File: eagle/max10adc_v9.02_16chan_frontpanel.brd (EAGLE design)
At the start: 79 x 65 mm, 106 parts, among them CN1 8p-2.54, X1 BU-SMA-V, X10 BU-SMA-V, X11 BU-SMA-V, X12 BU-SMA-V, X13 BU-SMA-V, X14 BU-SMA-V, X15 BU-SMA-V, X16 BU-SMA-V, X2 BU-SMA-V, X3 BU-SMA-V, X4 BU-SMA-V, X5 BU-SMA-V, X6 BU-SMA-V, X7 BU-SMA-V, X8 BU-SMA-V, X9 BU-SMA-V

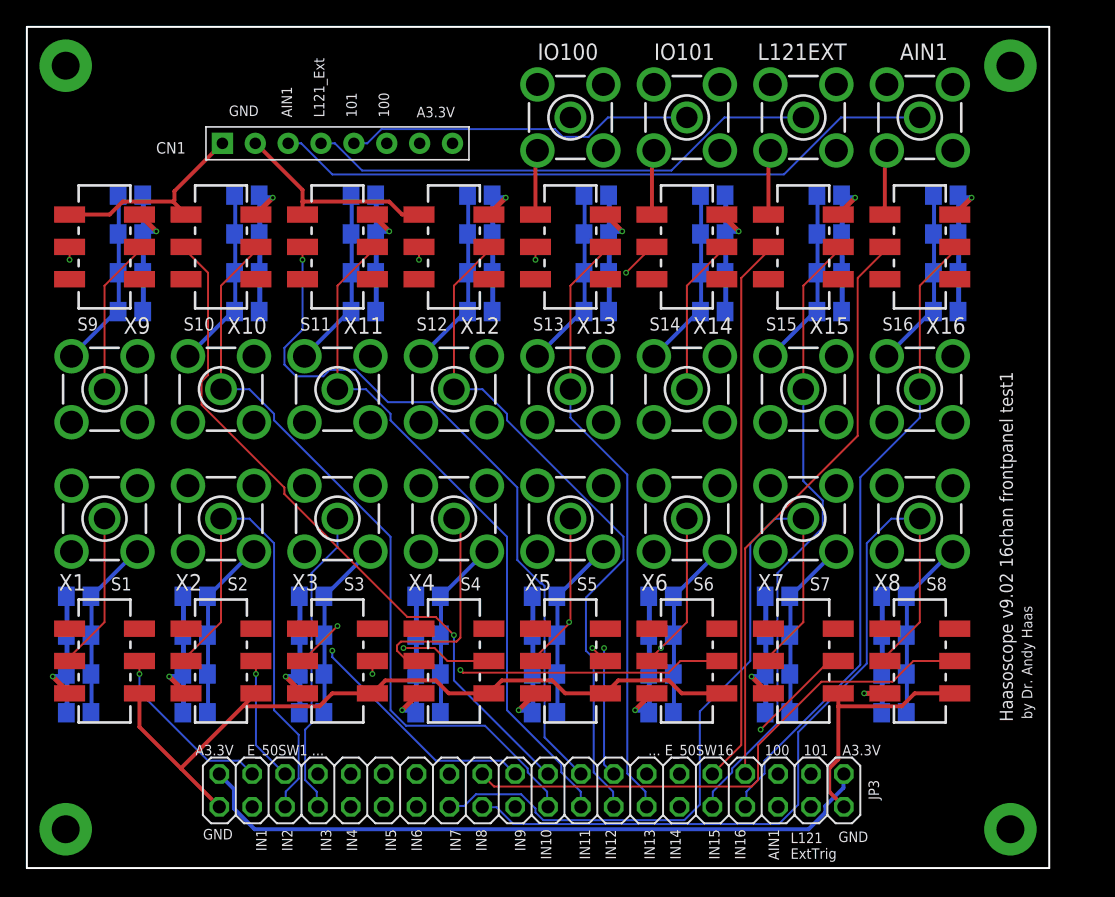
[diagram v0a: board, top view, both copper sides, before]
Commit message: back connectors
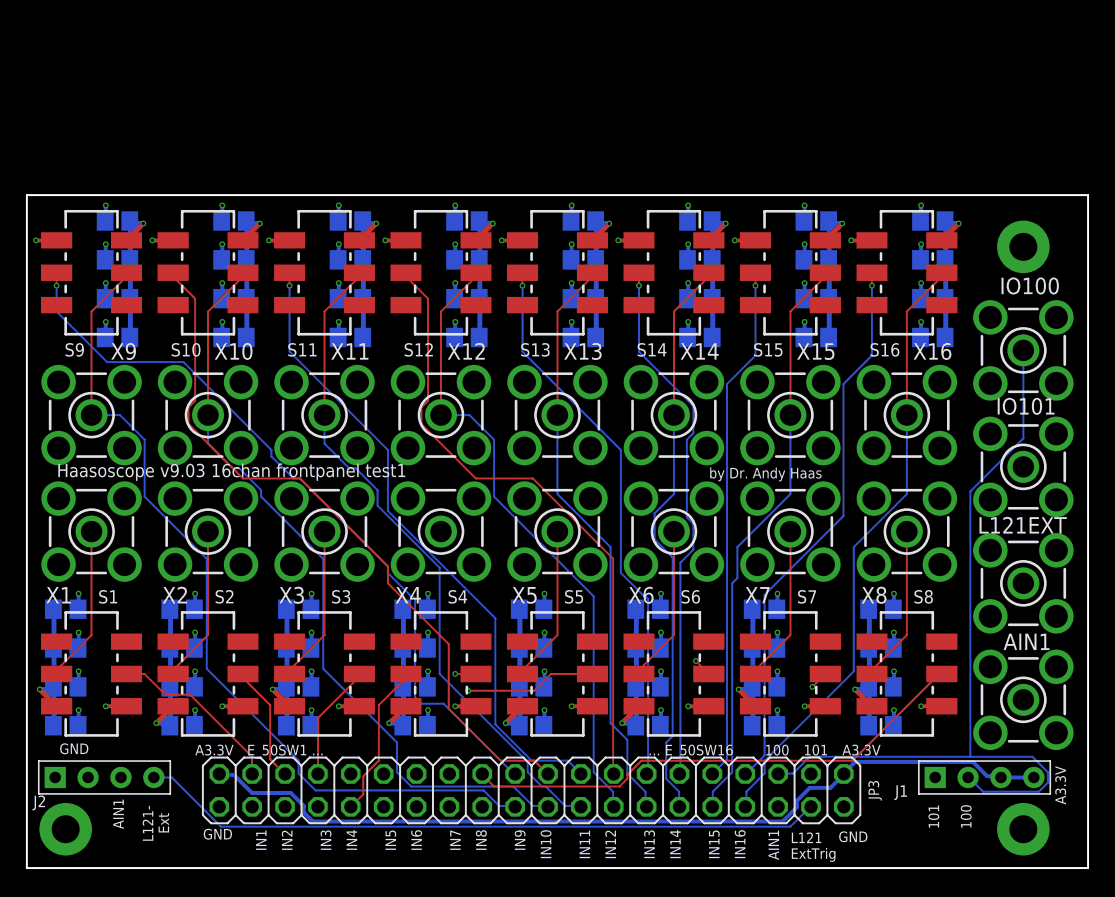
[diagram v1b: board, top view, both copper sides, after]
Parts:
- removed CN1: 8p-2.54, Seeed-Connector:H8-2.54
- removed H1: STANDOFF_ELECTRICAL, SparkFun-Hardware:STANDOFF-ELECTRICAL
- added J1, J2: 4p-2.54, Seeed-Connector:H4-2.54
- moved H2 75.3 mm to (77.0, 48.0)
- moved AIN1 45.7 mm to (77.0, 13.0)
- moved L121EXT 39.8 mm to (77.0, 22.0)
- moved IO100 39.4 mm to (77.0, 40.0)
- moved IO101 37.5 mm to (77.0, 31.0)
- moved R101 2.24 mm to (61.0, 41.0)
- moved R102 2.24 mm to (61.0, 44.0)
- moved R103 2.24 mm to (61.0, 47.0)
- moved R104 2.24 mm to (61.0, 50.0)
- moved R109 2.24 mm to (70.0, 41.0)
- moved R110 2.24 mm to (70.0, 44.0)
- moved R111 2.24 mm to (70.0, 47.0)
- moved R112 2.24 mm to (70.0, 50.0)
- moved R13 2.24 mm to (7.00, 41.0)
- moved R14 2.24 mm to (7.00, 44.0)
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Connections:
- net AIN1: now also J2.3; no longer CN1.3
- net GND: now also J2.1, J2.2; no longer CN1.1, CN1.2, H1.P1
- net IO_100: now also J1.2; no longer CN1.6
- net IO_101: now also J1.1; no longer CN1.5
- net L121: now also J2.4; no longer CN1.4
- net VCCA: now also J1.3, J1.4; no longer CN1.7, CN1.8
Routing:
- net GND: track 359.0 -> 105.6 mm, vias 0 -> 80
- net VCCA: track 111.3 -> 67.5 mm
- net IO_101: track 81.8 -> 38.4 mm
- net AIN1: track 114.1 -> 77.8 mm
- net L121: track 96.3 -> 80.2 mm
- net INJ14: track 55.1 -> 44.2 mm
- net INJ9: track 76.2 -> 65.5 mm
- net INJ7: track 60.1 -> 50.7 mm
- net IO_100: track 72.0 -> 62.7 mm
- net INJ8: track 65.0 -> 55.9 mm
- net E_50SW11: track 56.2 -> 49.7 mm
- net E_50SW13: track 48.4 -> 42.8 mm
- net E_50SW4: track 18.4 -> 12.9 mm
- net INJ4: track 42.6 -> 37.0 mm
- net E_50SW7: track 34.7 -> 40.1 mm
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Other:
- board size 79 x 65 mm -> 82 x 52 mm
- board text added: "Haasoscope v9.03 16chan frontpanel test1"
- board text added: "L121- Ext"
- board text removed: "Haasoscope v9.02 16chan frontpanel test1"
- board text removed: "L121_Ext"
